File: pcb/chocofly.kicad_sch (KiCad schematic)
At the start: 193 parts, among them P1 battery+, P2 battery-, SW1 SW_Push, SW11 SW_Push, SW12 SW_Push, SW13 SW_Push, SW14 SW_Push, SW15 SW_Push, SW16 SW_Push, SW17 SW_Push, SW18 SW_Push, SW19 SW_Push, SW2 SW_Push, SW20 SW_Push, SW21 SW_Push, SW22 SW_Push, SW23 SW_Push, SW24 SW_Push, SW25 SW_Push, SW26 SW_Push, SW27 SW_Push, SW28 SW_Push, SW29 SW_Push, SW3 SW_Push, SW30 SW_Push, SW31 SW_Push, SW32 SW_Push, SW33 SW_Push, SW34 SW_Push, SW35 SW_Push, SW36 SW_Push, SW37 SW_Push, SW38 SW_Push, SW39 SW_Push, SW4 SW_Push, SW40 SW_Push, SW41 SW_Push, SW42 SW_Push, SW43 SW_Push, SW44 SW_Push, SW45 SW_Push, SW46 SW_Push, SW47 SW_Push, SW48 SW_Push, SW49 SW_Push, SW5 SW_Push, SW50 SW_Push, SW51 SW_Push, SW52 SW_Push, SW53 SW_Push, SW54 SW_Push, SW55 SW_Push, SW56 SW_Push, SW57 SW_Push, SW58 SW_Push, SW59 SW_Push, SW6 SW_Push, SW60 SW_Push, SW61 SW_Push, SW62 Reset, SW63 Power, SW64 Power, SW7 SW_Push, SW8 SW_Push, SW9 SW_Push

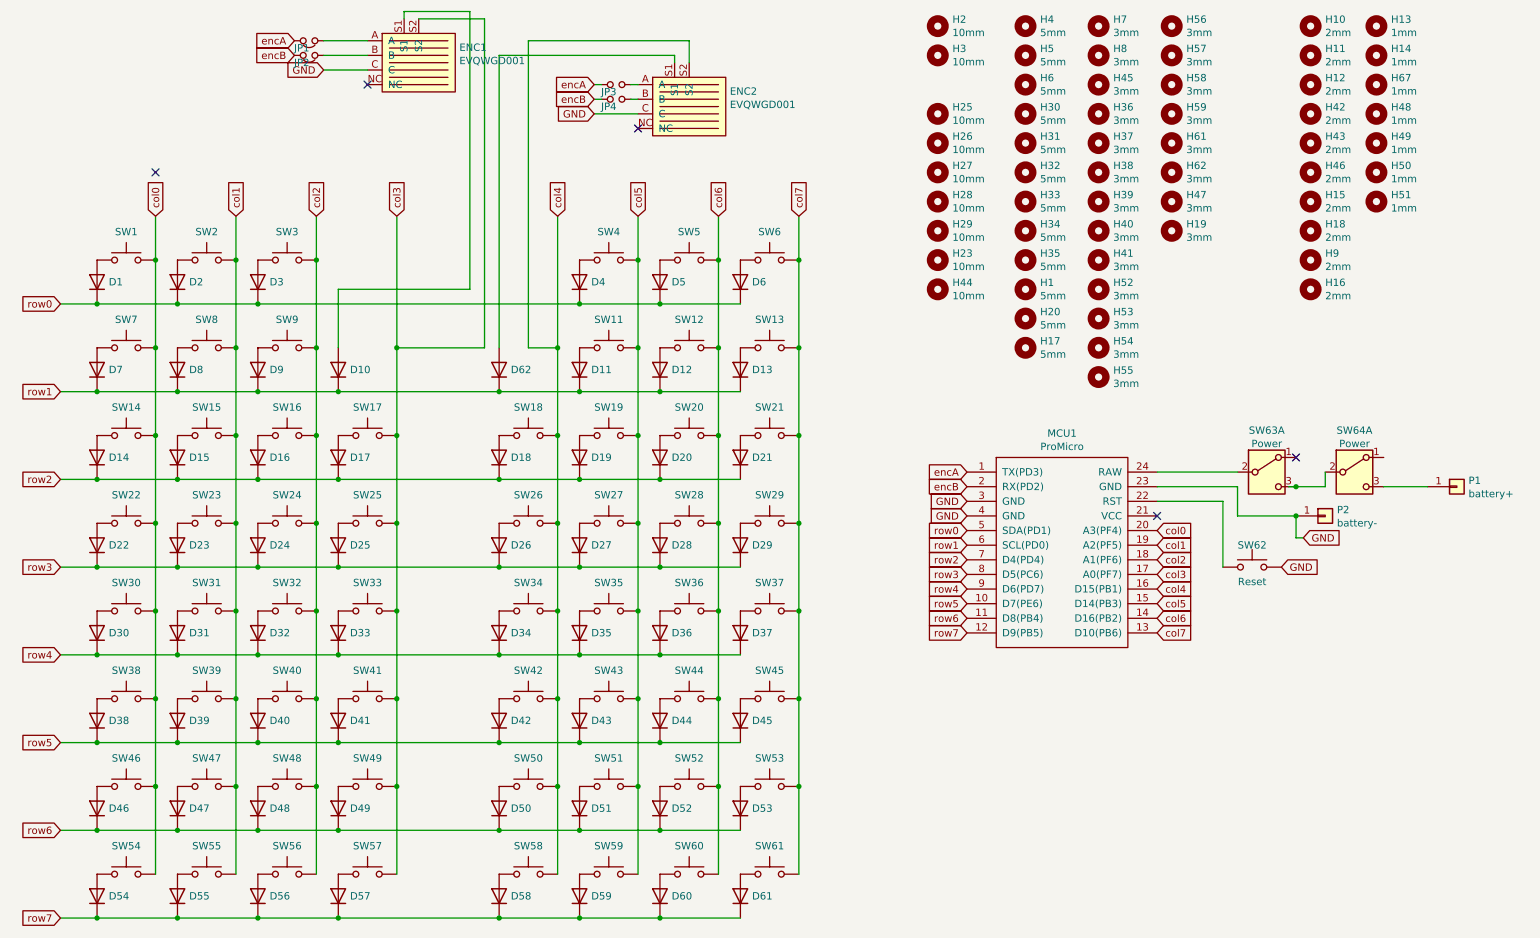
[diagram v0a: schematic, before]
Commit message: checks ok
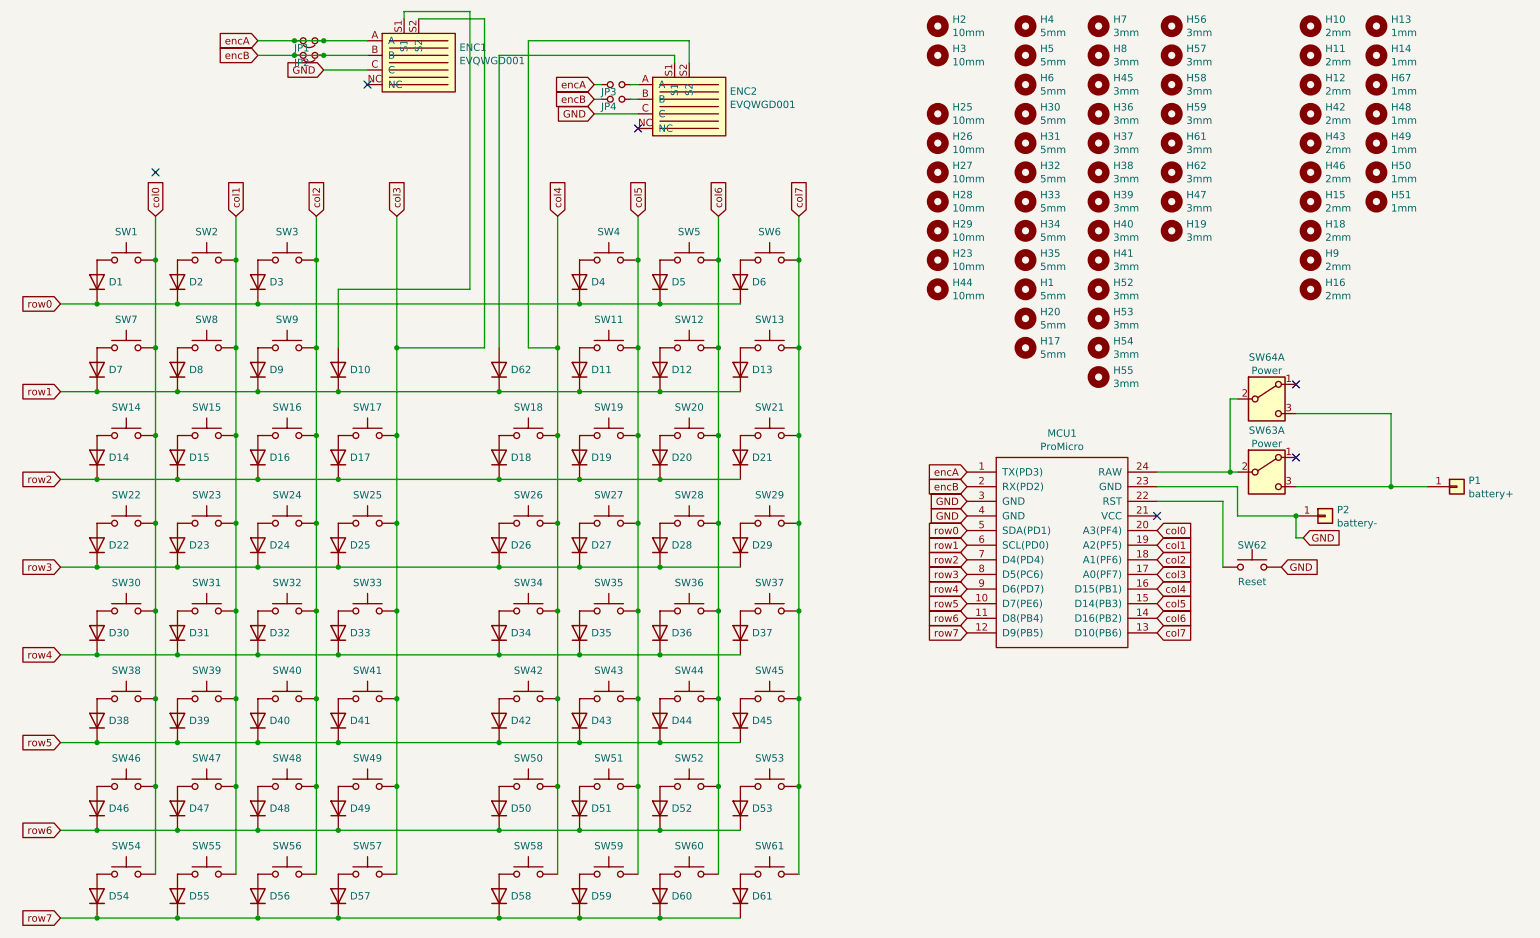
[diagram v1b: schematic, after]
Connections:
- net encA: now also ENC1.A, JP1.1
- net encB: now also ENC1.B, JP2.1
- net at P1.1 (Pin_1), SW64.3 (C): now also SW63.3 (C)
- net at MCU1.24 (RAW), SW63.2 (B): now also SW64.2 (B)
- no-connect marks 5 -> 6
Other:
- moved on the sheet: SW64A
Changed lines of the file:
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@@
 	)
 	(junction
-		(at 242.57 96.52)
-		(diameter 0)
-		(color 0 0 0 0)
-	)
-	(junction
 		(at 128.27 102.87)
 		(diameter 0)
@@
 	)
 	(junction
+		(at 68.58 21.59)
+		(diameter 0)
+		(color 0 0 0 0)
+	)
+	(junction
 		(at 48.26 80.01)
 		(diameter 0)
@@
 	)
 	(junction
+		(at 68.58 19.05)
+		(diameter 0)
+		(color 0 0 0 0)
+	)
+	(junction
 		(at 86.36 133.35)
 		(diameter 0)
@@
 	)
 	(junction
+		(at 231.14 93.98)
+		(diameter 0)
+		(color 0 0 0 0)
+	)
+	(junction
 		(at 156.21 72.39)
 		(diameter 0)
@@
 	)
 	(junction
+		(at 73.66 19.05)
+		(diameter 0)
+		(color 0 0 0 0)
+	)
+	(junction
 		(at 48.26 156.21)
 		(diameter 0)
@@
 	)
 	(junction
+		(at 73.66 21.59)
+		(diameter 0)
+		(color 0 0 0 0)
+	)
+	(junction
 		(at 114.3 87.63)
 		(diameter 0)
@@
 	)
 	(junction
+		(at 259.08 96.52)
+		(diameter 0)
+		(color 0 0 0 0)
+	)
+	(junction
 		(at 114.3 102.87)
 		(diameter 0)
@@
 	)
 	(no_connect
+		(at 242.57 78.74)
+	)
+	(no_connect
 		(at 128.27 34.29)
 	)
@@
 	(wire
 		(pts
-			(xy 247.65 96.52) (xy 247.65 93.98)
-		)
-		(stroke
-			(width 0)
-			(type default)
-		)
-	)
-	(wire
-		(pts
 			(xy 132.08 171.45) (xy 146.05 171.45)
 		)
@@
 	(wire
 		(pts
-			(xy 241.3 96.52) (xy 242.57 96.52)
+			(xy 156.21 87.63) (xy 156.21 102.87)
 		)
 		(stroke
@@
 	(wire
 		(pts
-			(xy 156.21 87.63) (xy 156.21 102.87)
+			(xy 259.08 96.52) (xy 265.43 96.52)
 		)
 		(stroke
@@
 	(wire
 		(pts
+			(xy 62.23 19.05) (xy 68.58 19.05)
+		)
+		(stroke
+			(width 0)
+			(type default)
+		)
+	)
+	(wire
+		(pts
 			(xy 27.94 64.77) (xy 34.29 64.77)
 		)
@@
 	(wire
 		(pts
+			(xy 231.14 81.28) (xy 231.14 93.98)
+		)
+		(stroke
+			(width 0)
+			(type default)
+		)
+	)
+	(wire
+		(pts
+			(xy 231.14 93.98) (xy 218.44 93.98)
+		)
+		(stroke
+			(width 0)
+			(type default)
+		)
+	)
+	(wire
+		(pts
 			(xy 132.08 110.49) (xy 146.05 110.49)
 		)
@@
 	(wire
 		(pts
+			(xy 242.57 96.52) (xy 259.08 96.52)
+		)
+		(stroke
+			(width 0)
+			(type default)
+		)
+	)
+	(wire
+		(pts
 			(xy 62.23 95.25) (xy 76.2 95.25)
 		)
@@
 	(wire
 		(pts
+			(xy 232.41 81.28) (xy 231.14 81.28)
+		)
+		(stroke
+			(width 0)
+			(type default)
+		)
+	)
+	(wire
+		(pts
 			(xy 48.26 80.01) (xy 62.23 80.01)
 		)
@@
 	(wire
 		(pts
-			(xy 257.81 96.52) (xy 265.43 96.52)
+			(xy 242.57 83.82) (xy 259.08 83.82)
 		)
 		(stroke
@@
 	(wire
 		(pts
+			(xy 68.58 19.05) (xy 73.66 19.05)
+		)
+		(stroke
+			(width 0)
+			(type default)
+		)
+	)
+	(wire
+		(pts
 			(xy 58.42 148.59) (xy 58.42 163.83)
 		)
@@
 	(wire
 		(pts
+			(xy 259.08 83.82) (xy 259.08 96.52)
+		)
+		(stroke
+			(width 0)
+			(type default)
+		)
+	)
+	(wire
+		(pts
+			(xy 62.23 21.59) (xy 68.58 21.59)
+		)
+		(stroke
+			(width 0)
+			(type default)
+		)
+	)
+	(wire
+		(pts
 			(xy 44.45 49.53) (xy 44.45 57.15)
 		)
@@
 	(wire
 		(pts
-			(xy 232.41 93.98) (xy 218.44 93.98)
+			(xy 232.41 93.98) (xy 231.14 93.98)
+		)
+		(stroke
+			(width 0)
+			(type default)
+		)
+	)
+	(wire
+		(pts
+			(xy 68.58 21.59) (xy 73.66 21.59)
 		)
 		(stroke
@@
 	(wire
 		(pts
-			(xy 242.57 96.52) (xy 247.65 96.52)
-		)
-		(stroke
-			(width 0)
-			(type default)
-		)
-	)
-	(wire
-		(pts
 			(xy 121.92 29.21) (xy 120.65 29.21)
 		)
@@
 	(global_label "encA"
 		(shape input)
-		(at 68.58 19.05 180)
+		(at 62.23 19.05 180)
 		(effects
 			(font
@@
 		)
 		(property "Intersheetrefs" "${INTERSHEET_REFS}"
-			(at 68.58 19.05 0)
+			(at 62.23 19.05 0)
 			(effects
 				(font
@@
 	(global_label "encB"
 		(shape input)
-		(at 68.58 21.59 180)
+		(at 62.23 21.59 180)
 		(effects
 			(font
@@
 		)
 		(property "Intersheetrefs" "${INTERSHEET_REFS}"
-			(at 68.58 21.59 0)
+			(at 62.23 21.59 0)
 			(effects
 				(font
@@
 	(symbol
 		(lib_id "Switch:SW_DPDT_x2")
-		(at 252.73 93.98 0)
+		(at 237.49 81.28 0)
 		(unit 1)
 		(exclude_from_sim no)
@@
 		(dnp no)
 		(property "Reference" "SW64"
-			(at 252.73 86.741 0)
+			(at 237.49 74.041 0)
 			(effects
 				(font
@@
 		)
 		(property "Value" "Power"
-			(at 252.73 89.0524 0)
+			(at 237.49 76.3524 0)
 			(effects
 				(font
@@
 		)
 		(property "Footprint" "footprints:Switch_MSK-12C01-07"
-			(at 252.73 93.98 0)
+			(at 237.49 81.28 0)
 			(effects
 				(font
@@
 		)
 		(property "Datasheet" "~"
-			(at 252.73 93.98 0)
+			(at 237.49 81.28 0)
 			(effects
 				(font
@@
 		)
 		(property "Description" ""
-			(at 252.73 93.98 0)
+			(at 237.49 81.28 0)
 			(effects
 				(font

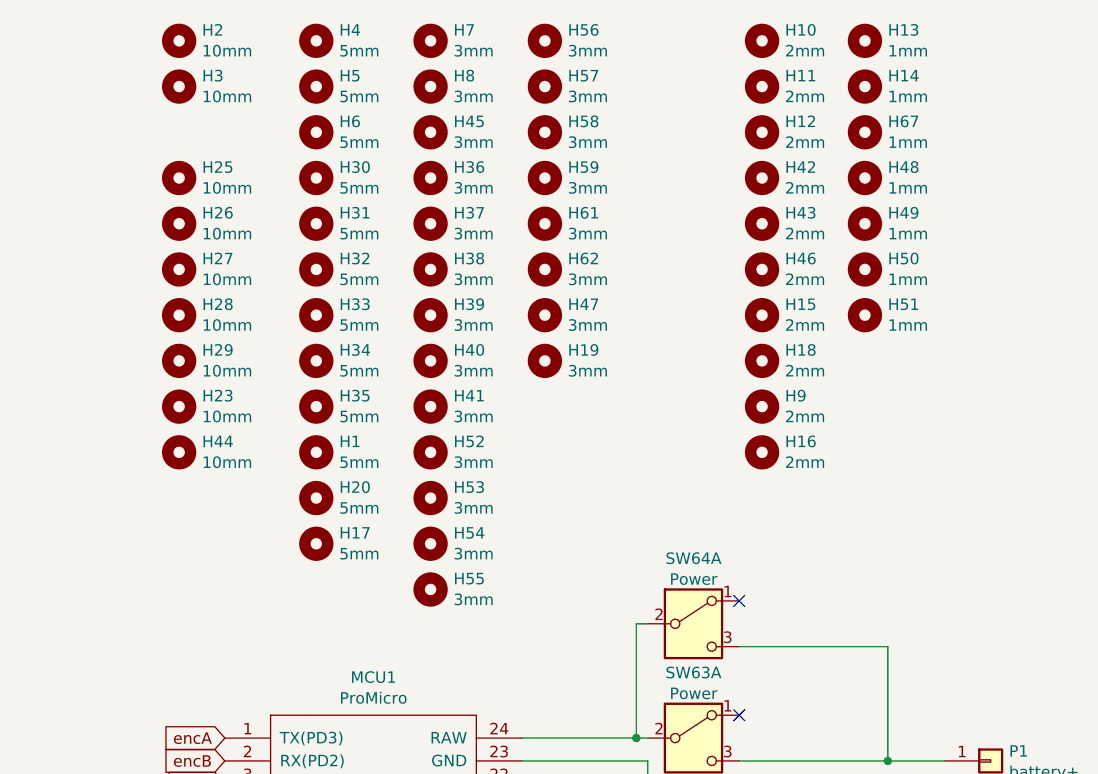
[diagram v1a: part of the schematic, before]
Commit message: fix
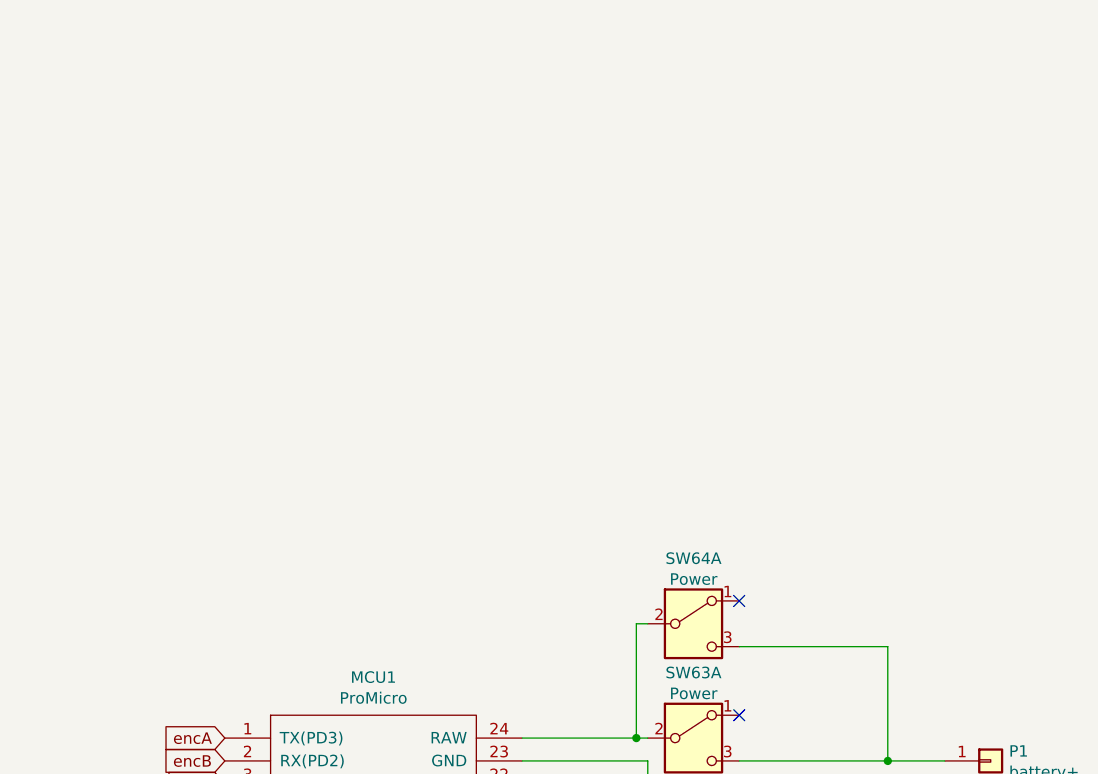
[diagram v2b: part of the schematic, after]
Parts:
- removed H1, H17, H20, H30, H31, H32, H33, H34, H35, H4, H5, H6: 5mm, footprints:hole_5mm, symbol Mechanical:MountingHole
- removed H10, H11, H12, H15, H16, H18, H42, H43, H46, H9: 2mm, footprints:hole_2mm, symbol Mechanical:MountingHole
- removed H13, H14, H48, H49, H50, H51, H67: 1mm, footprints:hole_1mm, symbol Mechanical:MountingHole
- removed H19, H36, H37, H38, H39, H40, H41, H45, H47, H52, H53, H54, H55, H56, H57, H58, H59, H61, H62, H7, H8: 3mm, footprints:hole_3mm, symbol Mechanical:MountingHole
- removed H2, H23, H25, H26, H27, H28, H29, H3, H44: 10mm, footprints:hole_10mm, symbol Mechanical:MountingHole
